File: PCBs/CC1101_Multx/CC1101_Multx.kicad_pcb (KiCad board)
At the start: 4 copper layers, 35.4 x 25.9 mm, 50 parts, among them IC1 CC1101RGPR, J1 MCU, J2 MCU, J3 MCU, J4 MCU, J5 MCU, J6 MCU, J7 MCU, J8 MCU, J9 MCU, U1 4259-63, U3 4259-63, Y1 XRCGB26M000F1S2BR0

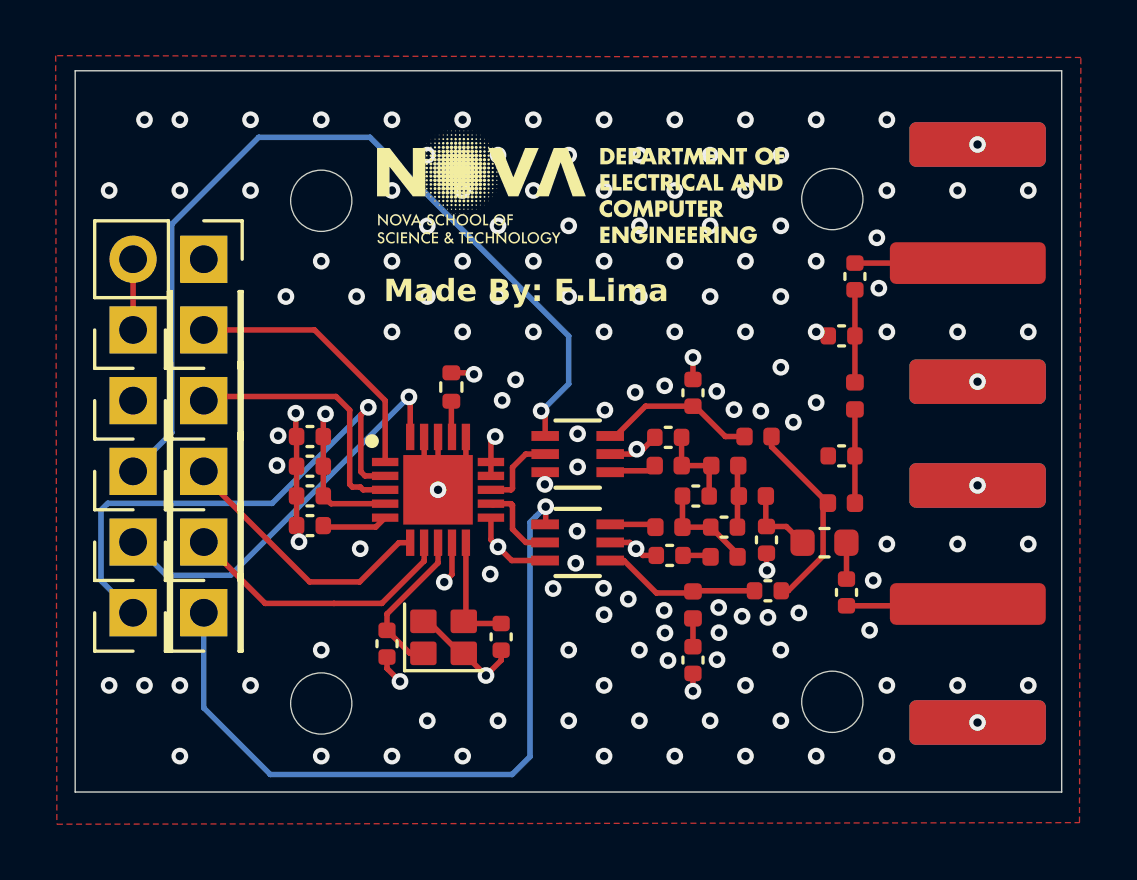
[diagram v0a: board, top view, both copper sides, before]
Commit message: symetric
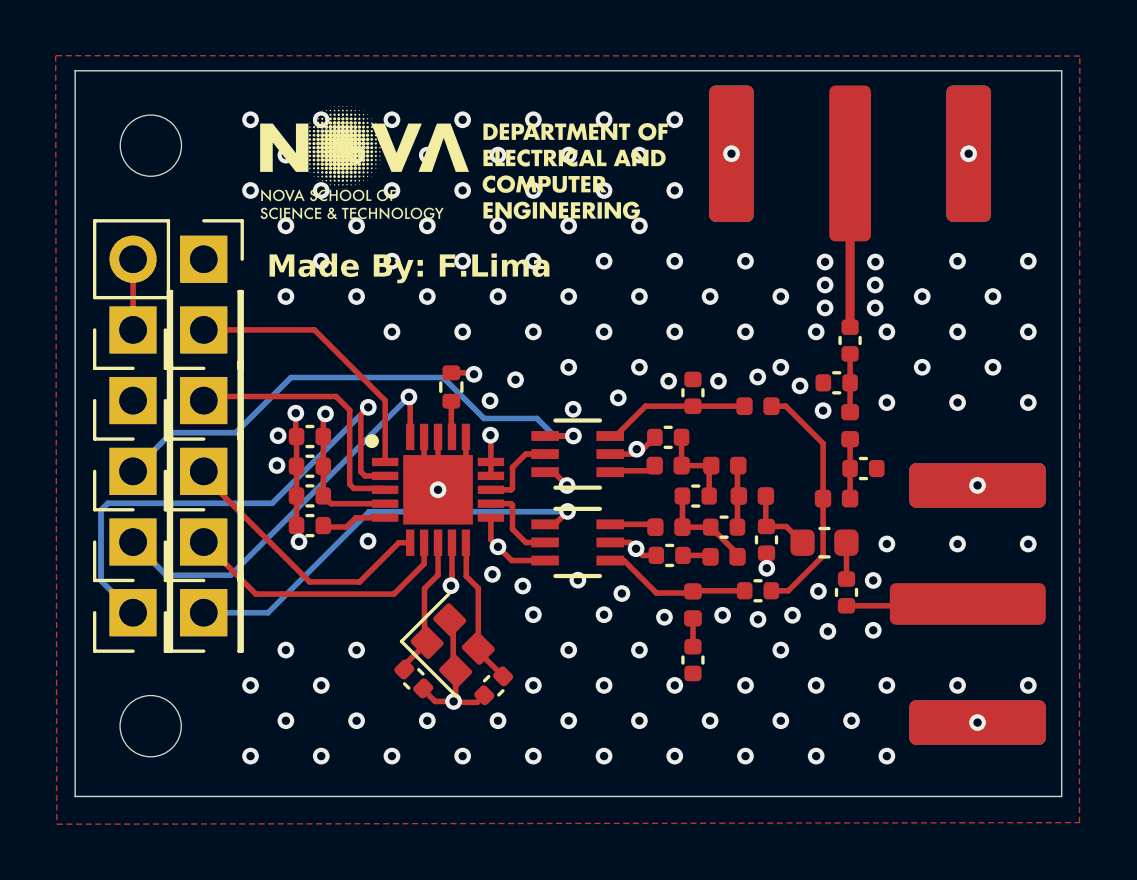
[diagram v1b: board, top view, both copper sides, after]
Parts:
- removed the REF** at (170.8, 71.4)
- removed the REF** at (170.8, 89.5)
- moved REF** 6.43 mm to (146.3, 69.5)
- moved REF** 6.18 mm to (146.3, 90.4)
- moved AE1 5.54 mm to (171.4, 70.2), turned to 90 degrees
- moved C125_1 2.31 mm to (171.4, 76.5)
- moved C5 1.78 mm to (158.6, 88.9), turned to 45 degrees
- moved C123_1 1.69 mm to (170.9, 78.0)
- moved C4 1.59 mm to (155.7, 88.7), turned to 135 degrees
- moved L131_1 1.09 mm to (168.1, 78.9)
- moved L123_1 1.08 mm to (171.4, 79.6)
- moved C122_1 0.91 mm to (171.9, 81.1), turned to 180 degrees
- moved Y1 0.44 mm to (157.1, 87.5), turned to -45 degrees
- moved C121_1 0.36 mm to (168.1, 85.5)
- moved L122_1 0.24 mm to (170.9, 82.2)
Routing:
- net Net-(J7-Pin_1): track 32.0 -> 19.1 mm
- net Net-(J8-Pin_1): track 26.3 -> 15.6 mm
- net /433_A: track 4.05 -> 5.95 mm
- net Net-(C121_1-Pad2): track 7.22 -> 8.83 mm
- net /AGND: track 24.8 -> 23.3 mm
- net Net-(IC1-XOSC_Q2): track 4.23 -> 5.46 mm
- net Net-(C123_1-Pad2): track 3.33 -> 2.09 mm
- net Net-(C122_1-Pad2): track 3.37 -> 2.13 mm
- net /AVDD: track 11.8 -> 12.4 mm
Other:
- board size 35.4 x 25.9 mm -> 35.4 x 26.1 mm
